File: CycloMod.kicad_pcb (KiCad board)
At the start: 4 copper layers, 22 x 22 mm, 71 parts, among them J1 MICROMOD-2222, U1 10CL010YM164, U2 W25Q128JVS, U3 1.2V, U4 RP2350_60QFN, U5 MIC5504-2.5YMT, Y1 ABM8-272-T3

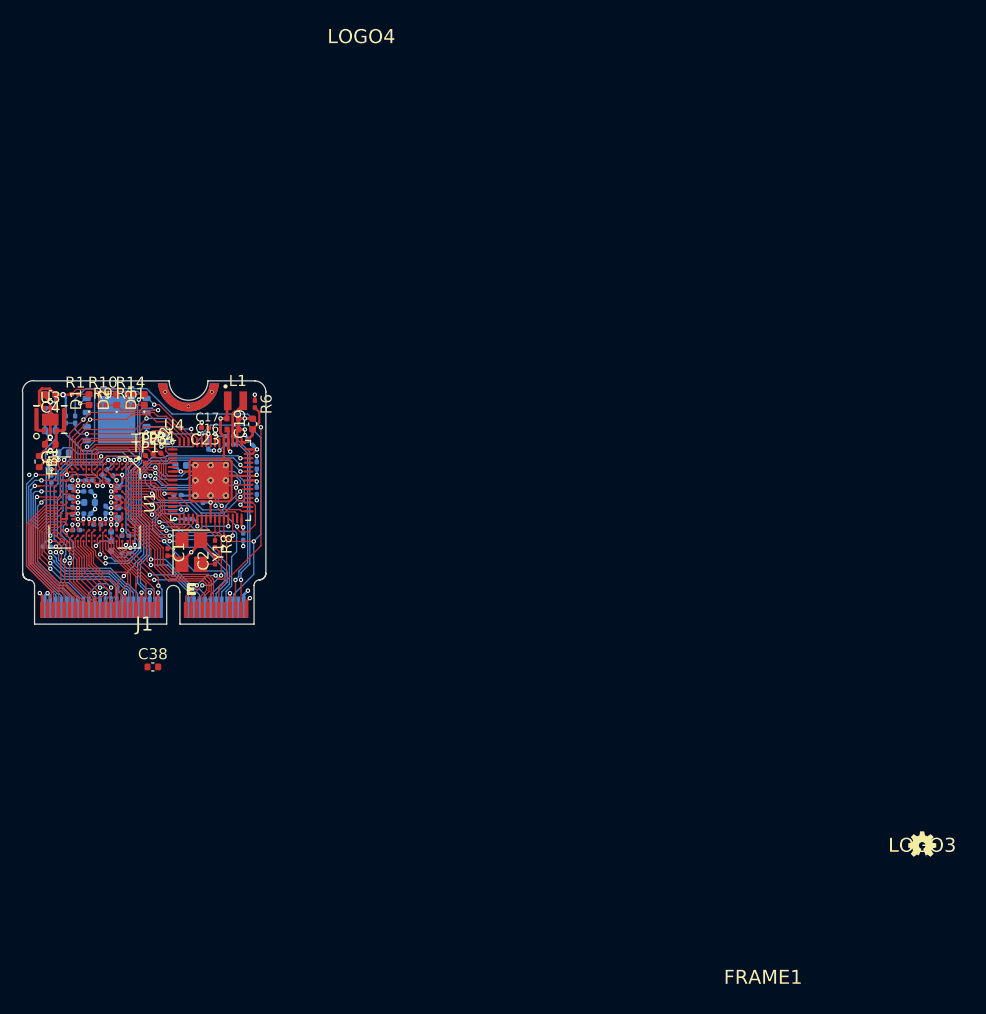
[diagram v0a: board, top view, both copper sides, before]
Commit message: started silkscreen cleanup, checking in prior to cardedge/outline update
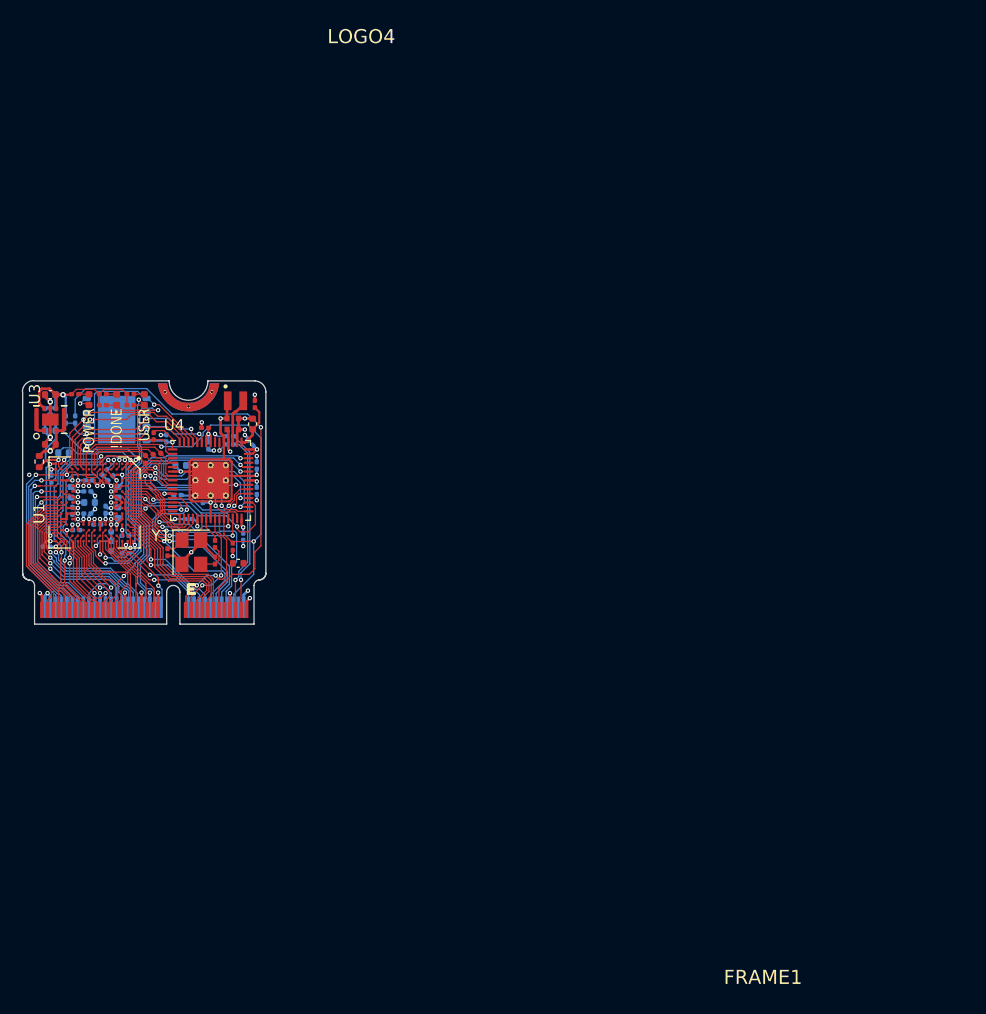
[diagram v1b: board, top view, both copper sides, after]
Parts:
- added R4: 10k, Resistor_SMD:R_0201_0603Metric, F.Cu at (156.5, 109.0)
- FB1: value FerriteBead_Small -> 120
- LOGO3: moved to B.Cu
- moved LOGO3 72.1 mm to (151.1, 111.2), turned to 180 degrees
- moved C38 12.1 mm to (157.0, 110.5)
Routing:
- net /CLKIN1: track 14.2 -> 13.3 mm
- net /~{BOOT}: track 38.3 -> 39.2 mm
- net +3V3: track 54.1 -> 54.6 mm, vias 19 -> 20
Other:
- board text added: "!DONE"
- board text added: "JT AS"
- board text added: "POWER"
- board text added: "USER"
